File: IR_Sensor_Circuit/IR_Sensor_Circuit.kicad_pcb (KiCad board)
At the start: 2 copper layers, 47.6 x 26.9 mm, 9 parts, among them J1 Conn_01x03_Pin, U1 LM358

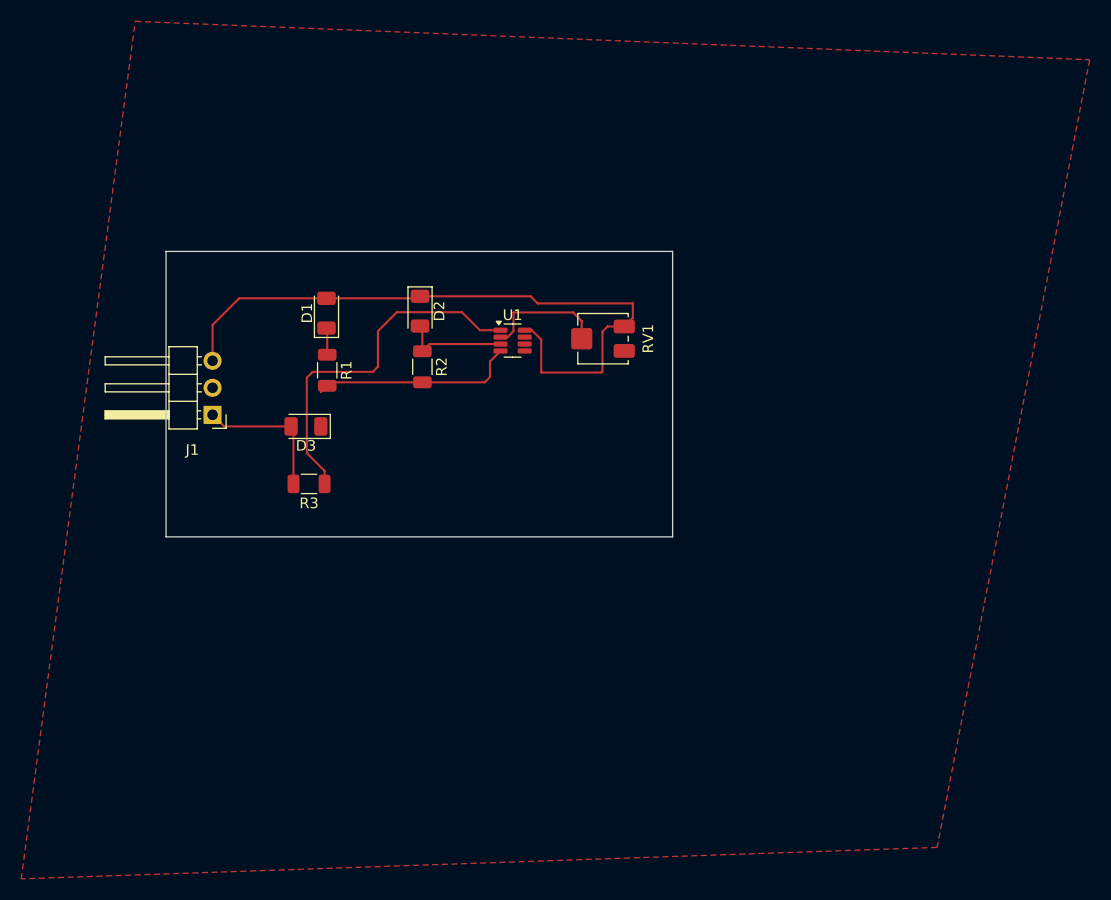
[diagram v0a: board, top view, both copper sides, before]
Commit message: IR Sensor
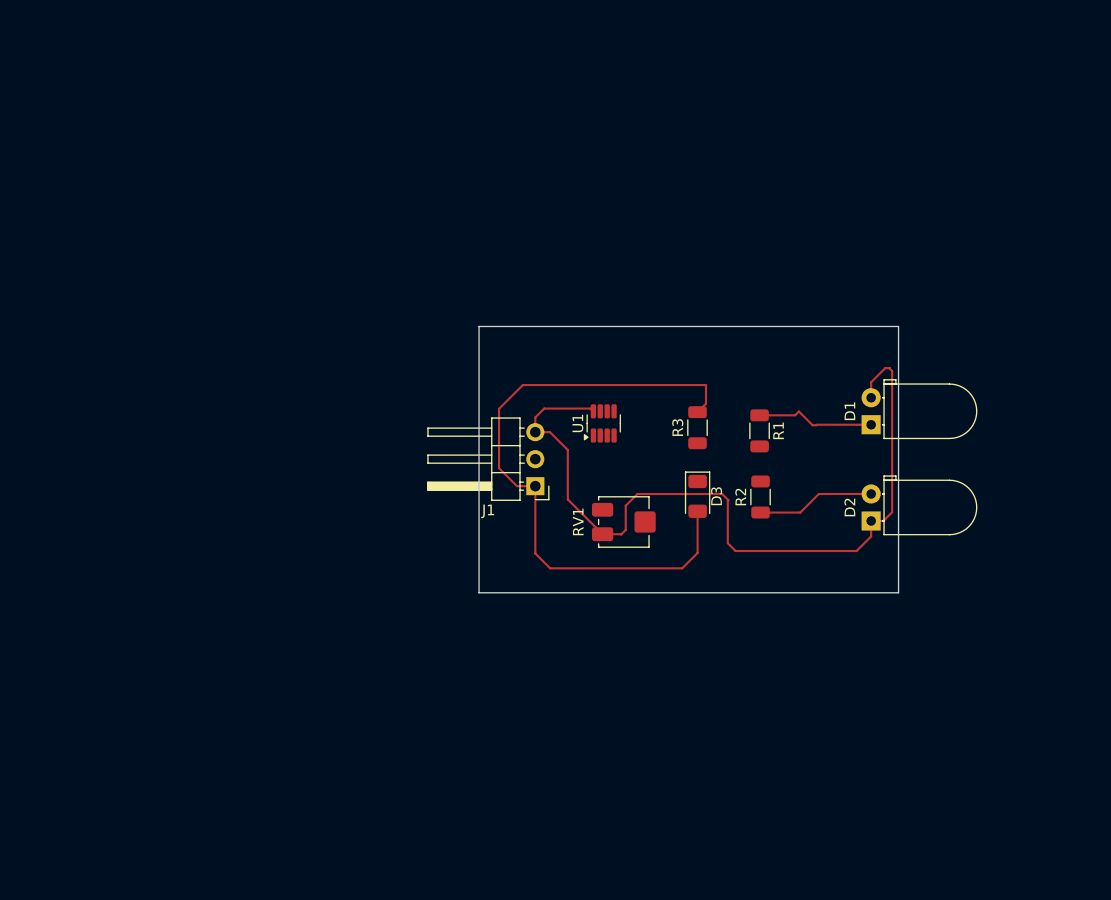
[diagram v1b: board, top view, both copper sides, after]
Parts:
- D1: footprint LED_SMD:LED_1206_3216Metric -> LED_THT:LED_D5.0mm_Horizontal_O1.27mm_Z3.0mm_IRBlack
- D2: footprint LED_SMD:LED_1206_3216Metric -> LED_THT:LED_D5.0mm_Horizontal_O1.27mm_Z3.0mm_IRGrey
- moved D1 52.3 mm to (121.8, 115.8)
- moved D2 46.8 mm to (121.8, 124.9), turned to 90 degrees
- moved R1 41.1 mm to (111.3, 116.4)
- moved D3 37.4 mm to (105.5, 122.6), turned to -90 degrees
- moved R3 36.9 mm to (105.5, 116.1), turned to 90 degrees
- moved R2 34.1 mm to (111.4, 122.6), turned to 90 degrees
- moved J1 31.1 mm to (90.2, 121.6)
- moved RV1 17.4 mm to (98.5, 125.0), turned to 90 degrees
- moved U1 11.6 mm to (96.7, 115.7), turned to 90 degrees
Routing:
- net /OUTPUT: track 13.3 -> 59.7 mm
- net Net-(R3-Pad1): track 34.1 -> 0.00 mm
- net /GND: track 19.4 -> 0.00 mm
- net /POT_V: track 11.6 -> 0.00 mm
- net /VCC: track 63.6 -> 74.9 mm
- net Net-(D1-K): track 2.54 -> 11.2 mm
- net /PHD_V: track 10.1 -> 11.1 mm
- removed copper zone on F.Cu, net /GND
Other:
- board size 47.6 x 26.9 mm -> 39.5 x 25 mm
